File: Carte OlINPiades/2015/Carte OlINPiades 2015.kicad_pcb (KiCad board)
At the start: 2 copper layers, 283 parts, among them U1 dsPIC33FJ128MC802, U2 LM7805, U3 LM2937-3.3

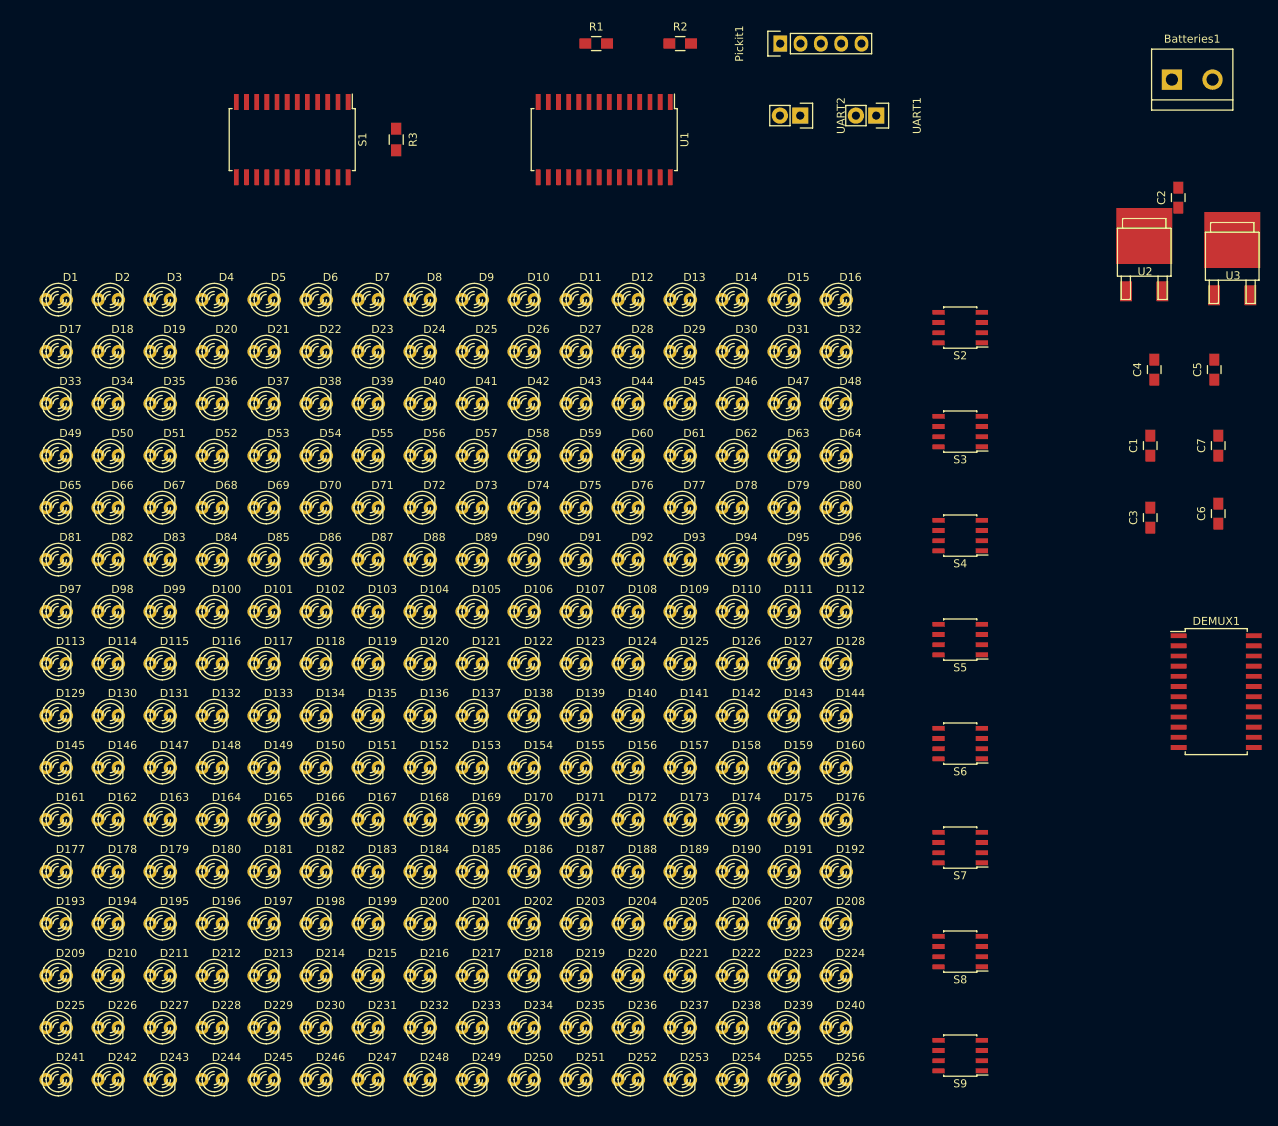
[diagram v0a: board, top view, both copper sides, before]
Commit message: retourne leds
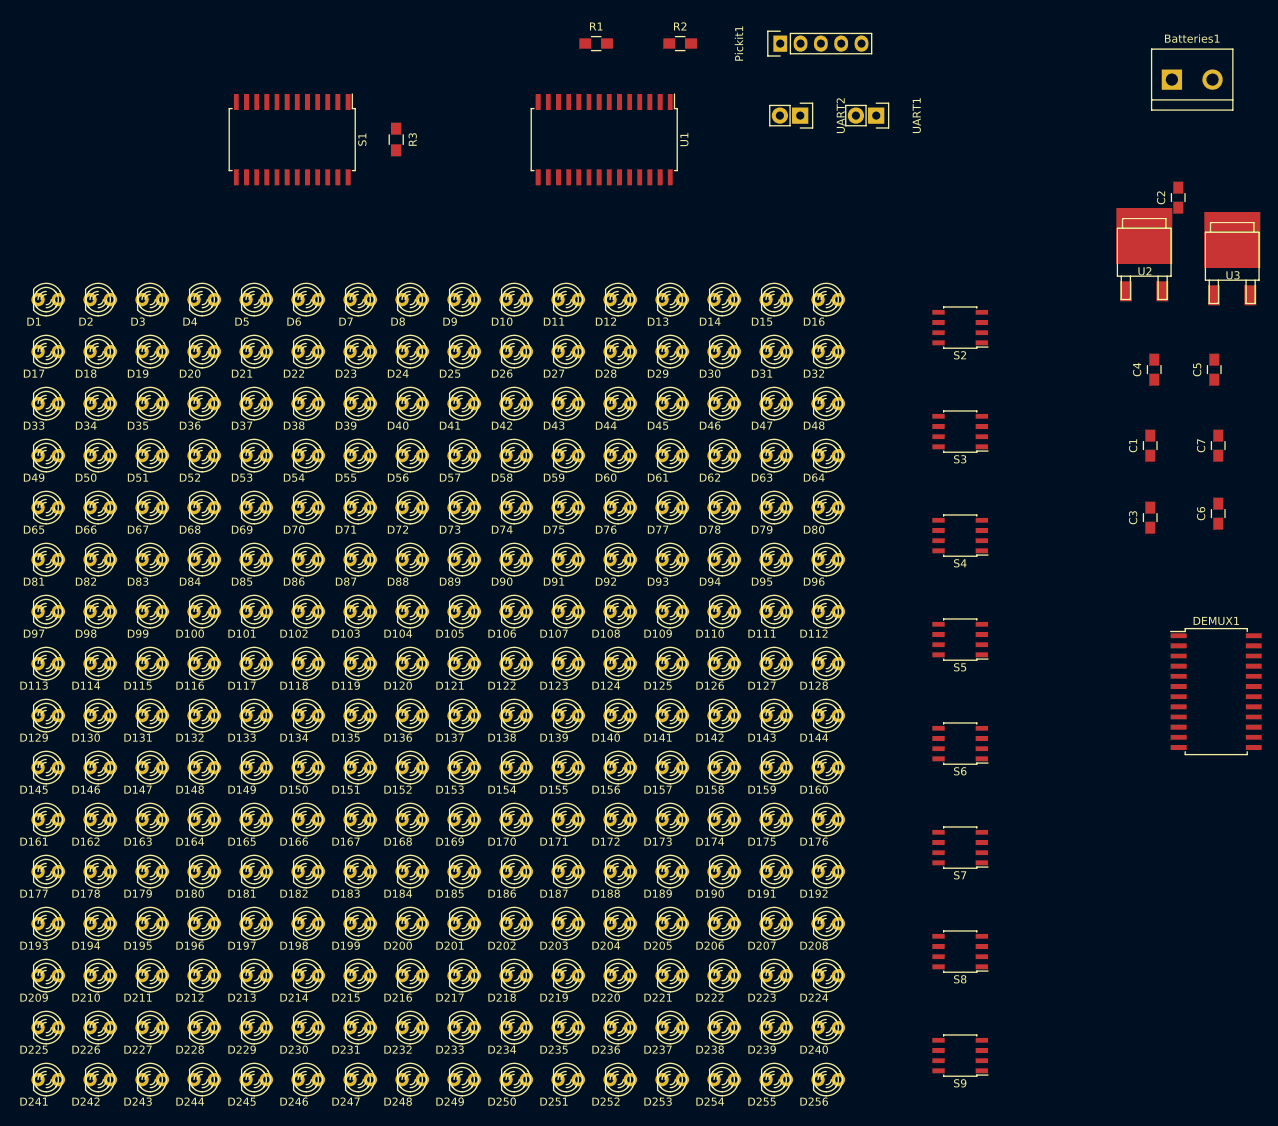
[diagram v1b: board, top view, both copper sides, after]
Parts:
- moved D1 1.00 mm to (47.5, 64.0), turned to 180 degrees
- moved D10 1.00 mm to (106.0, 64.0), turned to 180 degrees
- moved D100 1.00 mm to (67.0, 103.0), turned to 180 degrees
- moved D101 1.00 mm to (73.5, 103.0), turned to 180 degrees
- moved D102 1.00 mm to (80.0, 103.0), turned to 180 degrees
- moved D103 1.00 mm to (86.5, 103.0), turned to 180 degrees
- moved D104 1.00 mm to (93.0, 103.0), turned to 180 degrees
- moved D105 1.00 mm to (99.5, 103.0), turned to 180 degrees
- moved D106 1.00 mm to (106.0, 103.0), turned to 180 degrees
- moved D107 1.00 mm to (112.5, 103.0), turned to 180 degrees
- moved D108 1.00 mm to (119.0, 103.0), turned to 180 degrees
- moved D109 1.00 mm to (125.5, 103.0), turned to 180 degrees
- moved D11 1.00 mm to (112.5, 64.0), turned to 180 degrees
- moved D110 1.00 mm to (132.0, 103.0), turned to 180 degrees
- moved D111 1.00 mm to (138.5, 103.0), turned to 180 degrees
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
